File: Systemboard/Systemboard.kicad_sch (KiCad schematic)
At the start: 16 parts, among them J1 Conn_01x60, J108 Prog BT, U101 ESP32-WROOM-32E

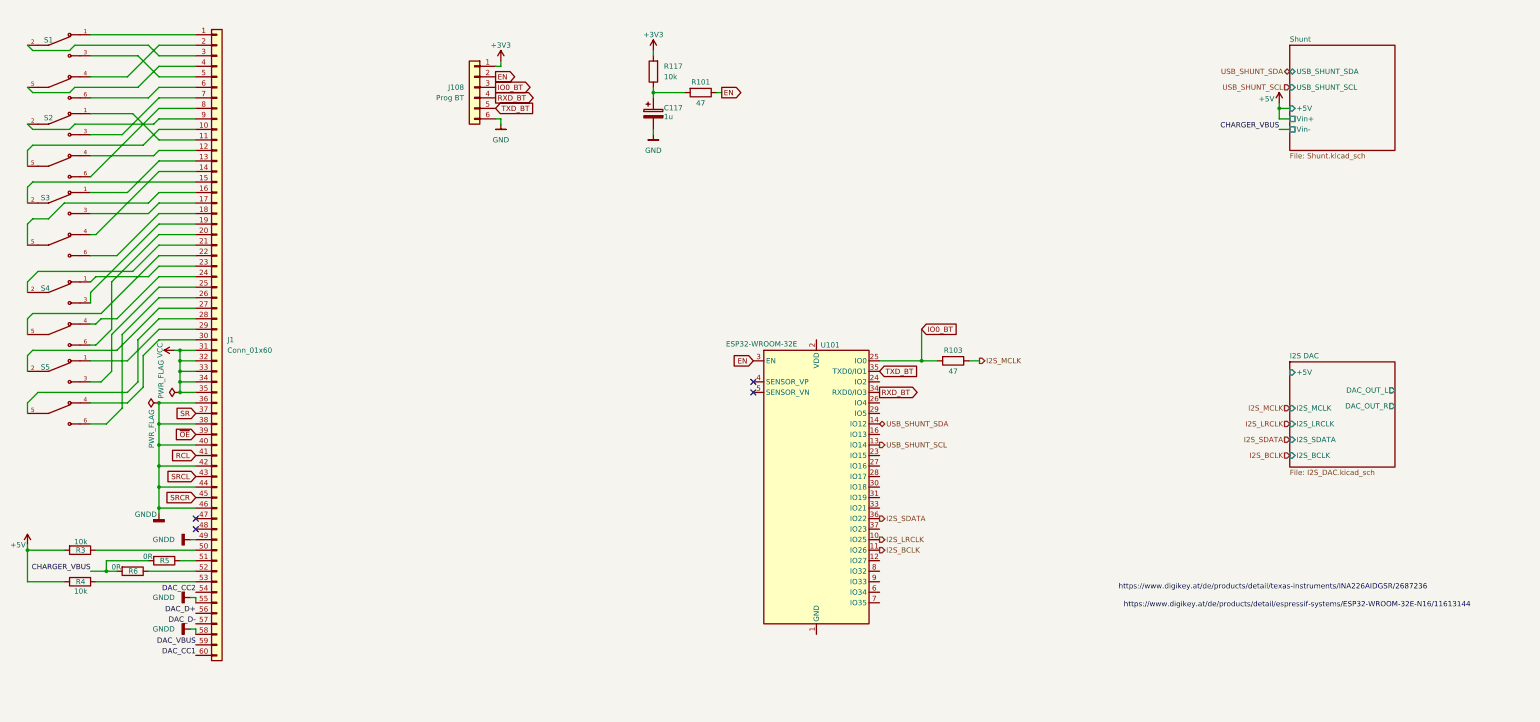
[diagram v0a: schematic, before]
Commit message: user save
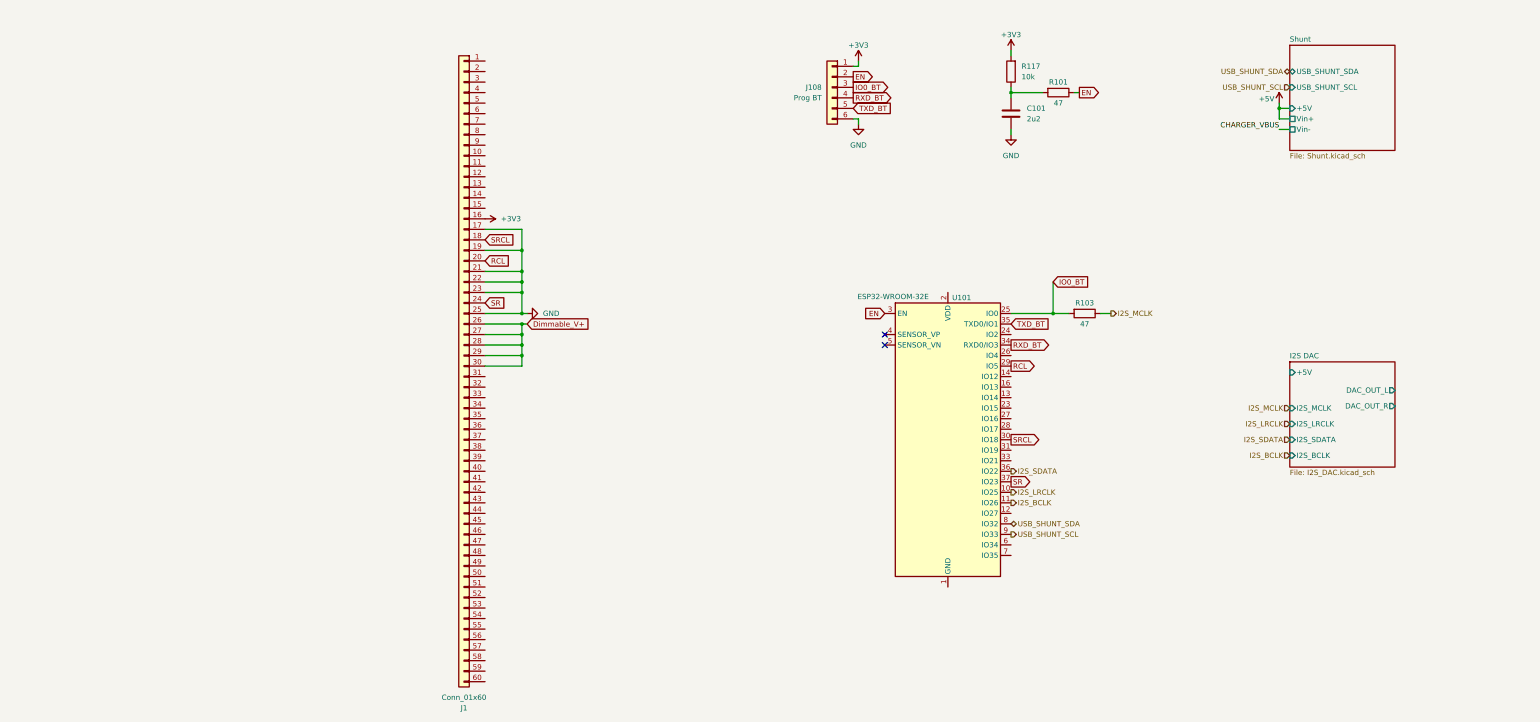
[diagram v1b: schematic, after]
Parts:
- removed C117: 1u, Capacitor_THT:CP_Radial_D5.0mm_P2.00mm, symbol Device:C_Polarized
- removed R3, R4: 10k, Resistor_THT:R_Axial_DIN0207_L6.3mm_D2.5mm_P10.16mm_Horizontal, symbol Device:R
- removed R5, R6: 0R, Resistor_THT:R_Axial_DIN0207_L6.3mm_D2.5mm_P10.16mm_Horizontal, symbol Device:R
- removed S1, S2, S3, S4, S5: TL2230EEF100, External_Parts:SW_TL2230EEF100, symbol External_Parts:TL2230EEF100
- added C101: 2u2, Capacitor_SMD:C_0603_1608Metric_Pad1.08x0.95mm_HandSolder, symbol Device:C
- J1: DigiKey Part # (none) -> 900-2004850460CT-ND
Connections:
- net +3V3: now also J1.16 (Pin_16)
- net GND: now also J1.17 (Pin_17), J1.19 (Pin_19), J1.21 (Pin_21), J1.22 (Pin_22), J1.23 (Pin_23), J1.25 (Pin_25), C101.2
- net RCL: now also J1.20 (Pin_20), U101.29 (IO5); no longer J1.41 (Pin_41)
- net SR: now also J1.24 (Pin_24), U101.37 (IO23); no longer J1.37 (Pin_37)
- net SRCL: now also J1.18 (Pin_18), U101.30 (IO18); no longer J1.43 (Pin_43)
- net USB_SHUNT_SCL: now also U101.9 (IO33); no longer U101.13 (IO14)
- net USB_SHUNT_SDA: now also U101.8 (IO32); no longer U101.14 (IO12)
- net Dimmable_V+: now reaches J1.29 (Pin_29)
- net Dimmable_V+: now also J1.26 (Pin_26), J1.27 (Pin_27), J1.28 (Pin_28), J1.30 (Pin_30)
- net at R101.2, R117.1: now also C101.1
- net DAC_CC1: no longer names the net of J1.60 (Pin_60)
- net DAC_CC2: no longer names the net of J1.54 (Pin_54)
- net DAC_D+: no longer names the net of J1.56 (Pin_56)
- net DAC_D-: no longer names the net of J1.57 (Pin_57)
- net DAC_VBUS: no longer names the net of J1.59 (Pin_59)
- removed net GNDD: J1.36 (Pin_36), J1.38 (Pin_38), J1.40 (Pin_40), J1.42 (Pin_42), J1.44 (Pin_44), J1.46 (Pin_46), J1.49 (Pin_49), J1.55 (Pin_55), J1.58 (Pin_58)
- net SRCR: no longer names the net of J1.45 (Pin_45)
- removed net VCC: J1.31 (Pin_31), J1.32 (Pin_32), J1.33 (Pin_33), J1.34 (Pin_34), J1.35 (Pin_35)
- net ~{OE}: no longer names the net of J1.39 (Pin_39)
- no-connect marks 4 -> 2
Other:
- note removed: "https://www.digikey.at/de/products/detail/espressif-systems/ESP32-WROOM-32E-N16/11613144"
- note removed: "https://www.digikey.at/de/products/detail/texas-instruments/INA226AIDGSR/2687236"
- moved on the sheet: J1, J108, R101, R103, R117, U101

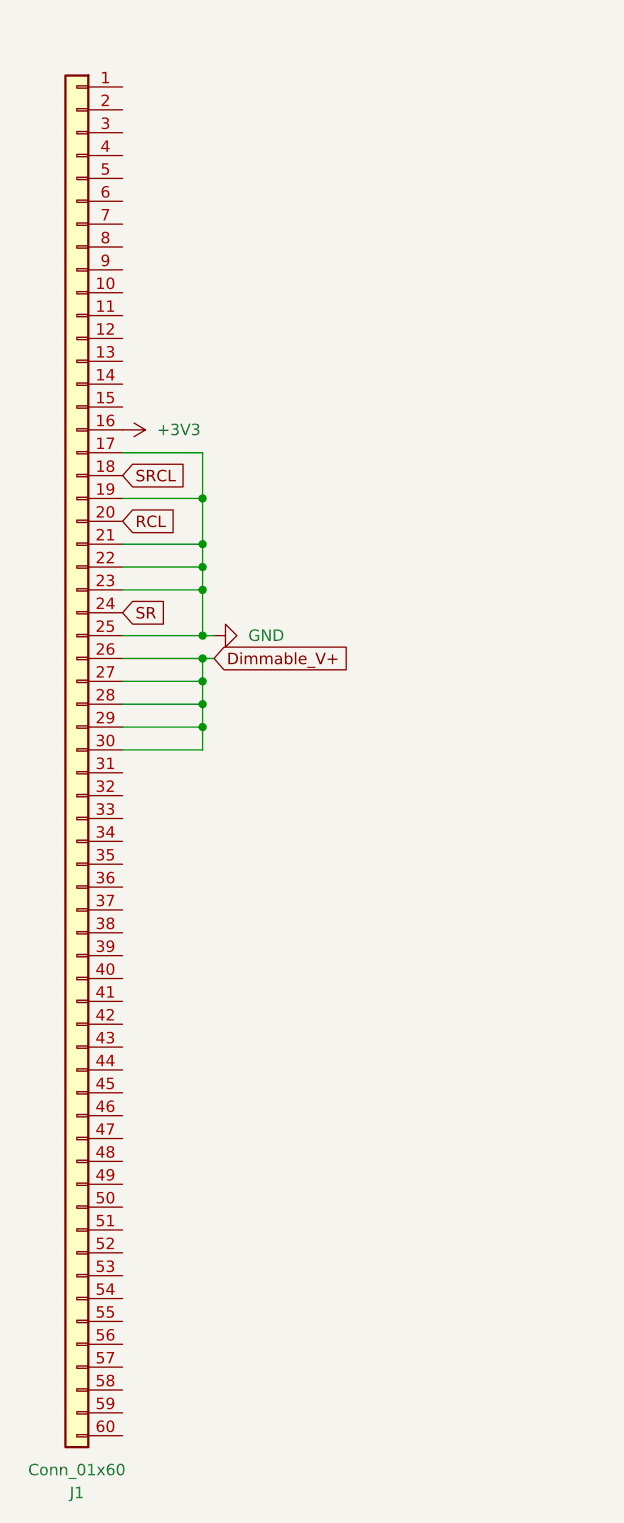
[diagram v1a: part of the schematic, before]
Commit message: Update Systemboard.kicad_sch
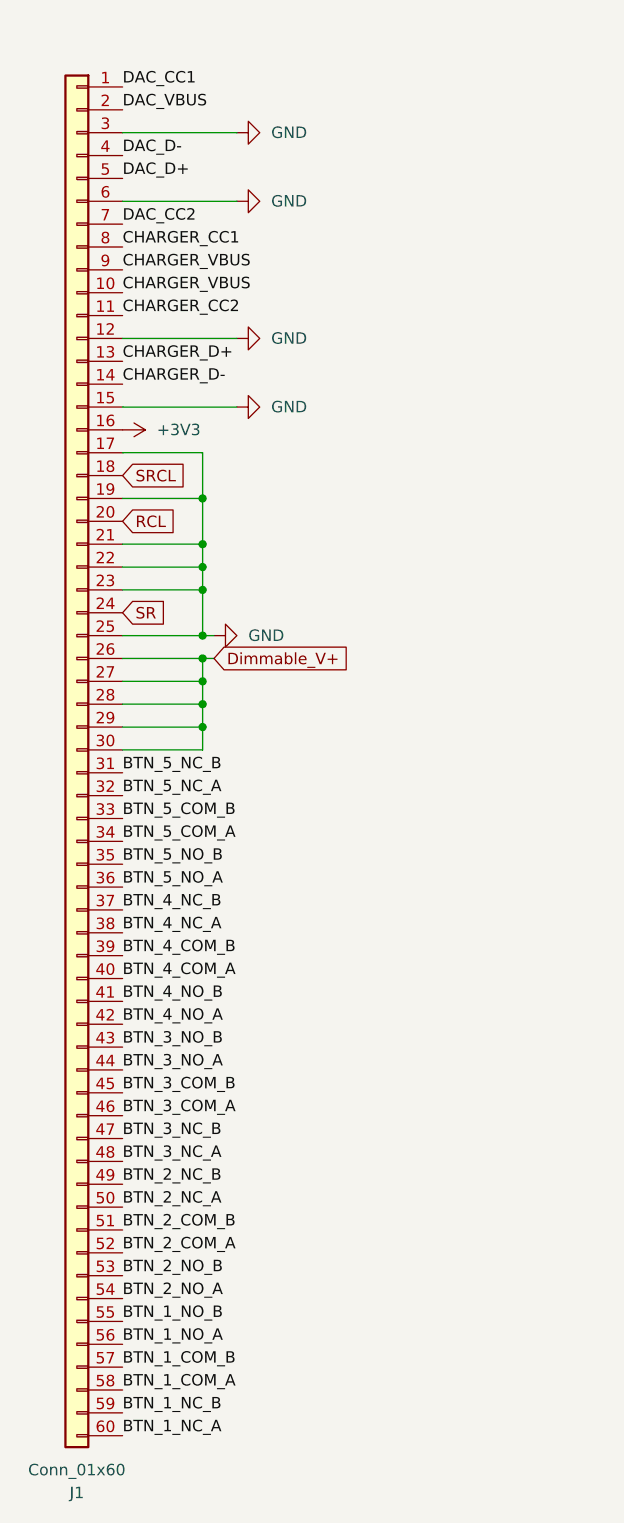
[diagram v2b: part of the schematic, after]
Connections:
- net CHARGER_VBUS: now also J1.10 (Pin_10), J1.9 (Pin_9)
- net GND: now also J1.12 (Pin_12), J1.15 (Pin_15), J1.3 (Pin_3), J1.6 (Pin_6)
- net DAC_CC1: now reaches J1.1 (Pin_1)
- net CHARGER_CC2: now reaches J1.11 (Pin_11)
- net CHARGER_D+: now reaches J1.13 (Pin_13)
- net CHARGER_D-: now reaches J1.14 (Pin_14)
- net DAC_VBUS: now reaches J1.2 (Pin_2)
- net BTN_5_NC_B: now reaches J1.31 (Pin_31)
- net BTN_5_NC_A: now reaches J1.32 (Pin_32)
- net BTN_5_COM_B: now reaches J1.33 (Pin_33)
- net BTN_5_COM_A: now reaches J1.34 (Pin_34)
- net BTN_5_NO_B: now reaches J1.35 (Pin_35)
- net BTN_5_NO_A: now reaches J1.36 (Pin_36)
- net BTN_4_NC_B: now reaches J1.37 (Pin_37)
- net BTN_4_NC_A: now reaches J1.38 (Pin_38)
- net BTN_4_COM_B: now reaches J1.39 (Pin_39)
- net DAC_D-: now reaches J1.4 (Pin_4)
- net BTN_4_COM_A: now reaches J1.40 (Pin_40)
- net BTN_4_NO_B: now reaches J1.41 (Pin_41)
- net BTN_4_NO_A: now reaches J1.42 (Pin_42)
- net BTN_3_NO_B: now reaches J1.43 (Pin_43)
- net BTN_3_NO_A: now reaches J1.44 (Pin_44)
- net BTN_3_COM_B: now reaches J1.45 (Pin_45)
- net BTN_3_COM_A: now reaches J1.46 (Pin_46)
- net BTN_3_NC_B: now reaches J1.47 (Pin_47)
- net BTN_3_NC_A: now reaches J1.48 (Pin_48)
- net BTN_2_NC_B: now reaches J1.49 (Pin_49)
- net DAC_D+: now reaches J1.5 (Pin_5)
- net BTN_2_NC_A: now reaches J1.50 (Pin_50)
- net BTN_2_COM_B: now reaches J1.51 (Pin_51)
- net BTN_2_COM_A: now reaches J1.52 (Pin_52)
- net BTN_2_NO_B: now reaches J1.53 (Pin_53)
- net BTN_2_NO_A: now reaches J1.54 (Pin_54)
- net BTN_1_NO_B: now reaches J1.55 (Pin_55)
- net BTN_1_NO_A: now reaches J1.56 (Pin_56)
- net BTN_1_COM_B: now reaches J1.57 (Pin_57)
- net BTN_1_COM_A: now reaches J1.58 (Pin_58)
- net BTN_1_NC_B: now reaches J1.59 (Pin_59)
- net BTN_1_NC_A: now reaches J1.60 (Pin_60)
- net DAC_CC2: now reaches J1.7 (Pin_7)
- net CHARGER_CC1: now reaches J1.8 (Pin_8)

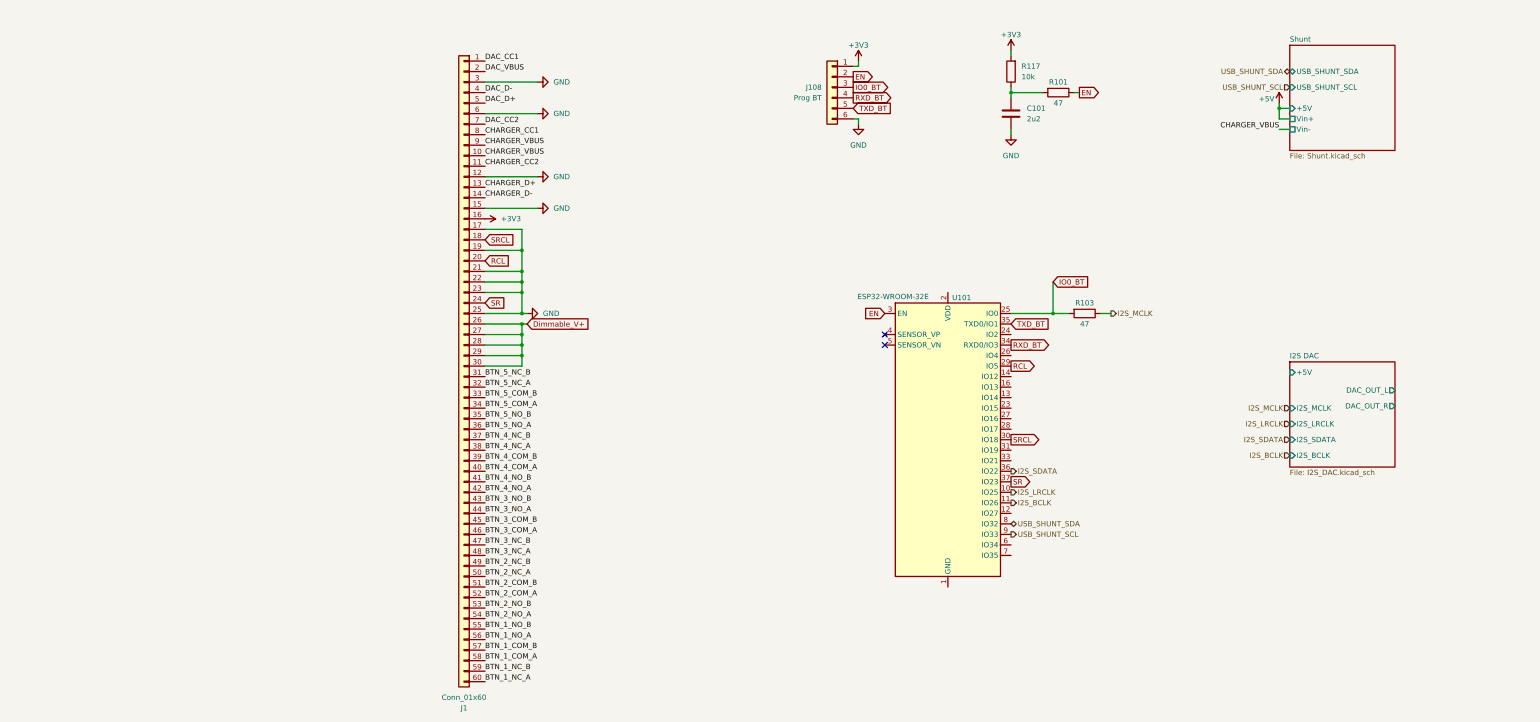
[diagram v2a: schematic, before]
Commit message: Update Systemboard.kicad_sch
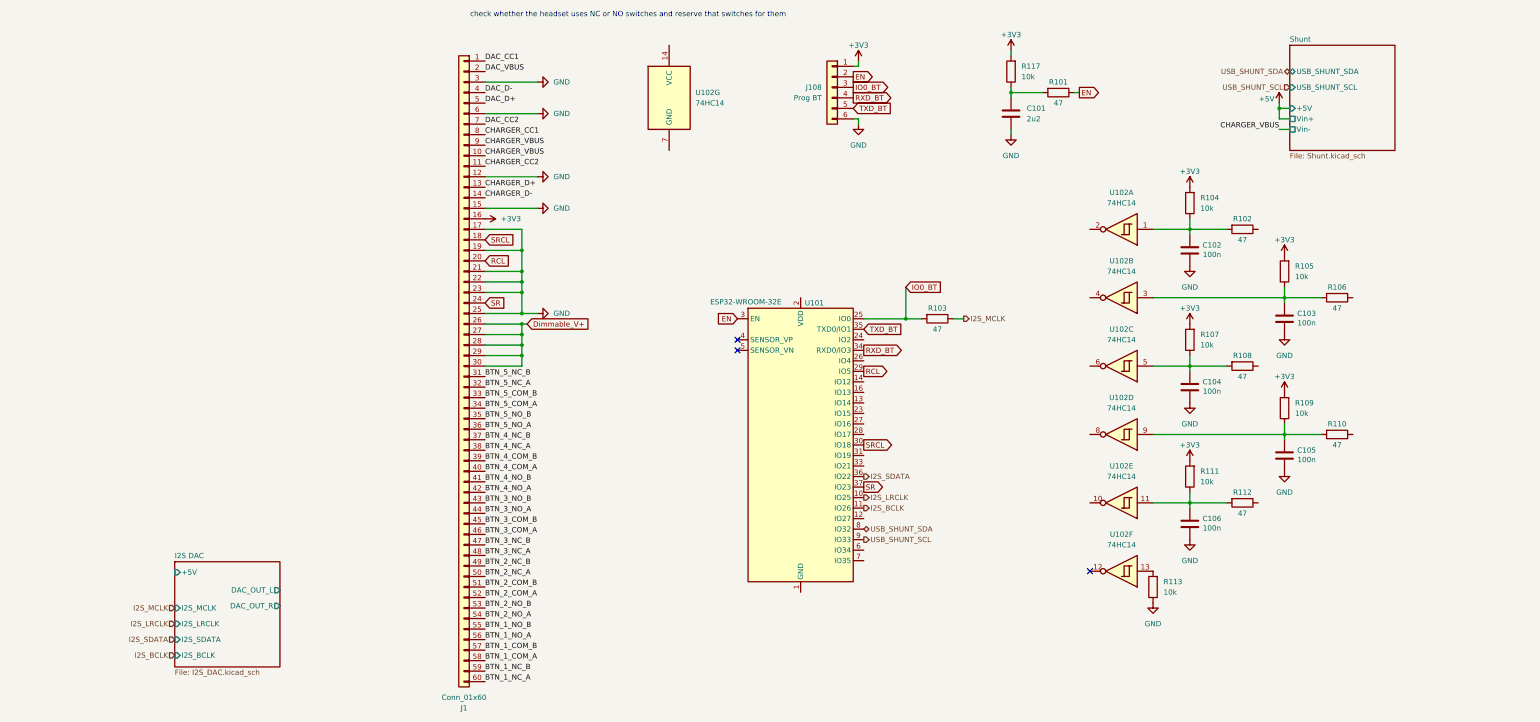
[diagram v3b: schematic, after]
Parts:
- added C102, C103, C104, C105, C106: 100n, Capacitor_SMD:C_0805_2012Metric_Pad1.18x1.45mm_HandSolder, symbol Device:C
- added R102, R106, R108, R110, R112: 47, Resistor_SMD:R_0402_1005Metric_Pad0.72x0.64mm_HandSolder, symbol Device:R
- added R104, R105, R107, R109, R111, R113: 10k, Resistor_SMD:R_0402_1005Metric_Pad0.72x0.64mm_HandSolder, symbol Device:R
- added U102: 74HC14, Package_SO:SOIC-14_3.9x8.7mm_P1.27mm, symbol 74xx:74HC14
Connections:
- net +3V3: now also R104.2, R105.2, R107.2, R109.2, R111.2
- net GND: now also C102.2, C103.2, C104.2, C105.2, C106.2, R113.1
- new net: C106.1, R111.1, R112.2, U102.11
- new net: C103.1, R105.1, R106.2, U102.3
- new net: C105.1, R109.1, R110.2, U102.9
- new net: C104.1, R107.1, R108.2, U102.5
- new net: C102.1, R102.2, R104.1, U102.1
- new net: R113.2, U102.13
- no-connect marks 2 -> 3
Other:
- note added: "check whether the headset uses NC or NO switches and reserve that switches for them"
- moved on the sheet: R103, U101
